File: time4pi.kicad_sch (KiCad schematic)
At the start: 17 parts, among them J1 Raspberry_Pi_2_3, J2 Conn_02x03_Odd_Even, J3 Conn_Coaxial_Small, J4 Conn_Coaxial_Small, J5 RFShield_OnePiece, Q3 BFR92, Q4 BFR92, U1 ECOC 7050, U2 HMC361S8G/361S8GE, U3 ADF4158, U4 AB0805

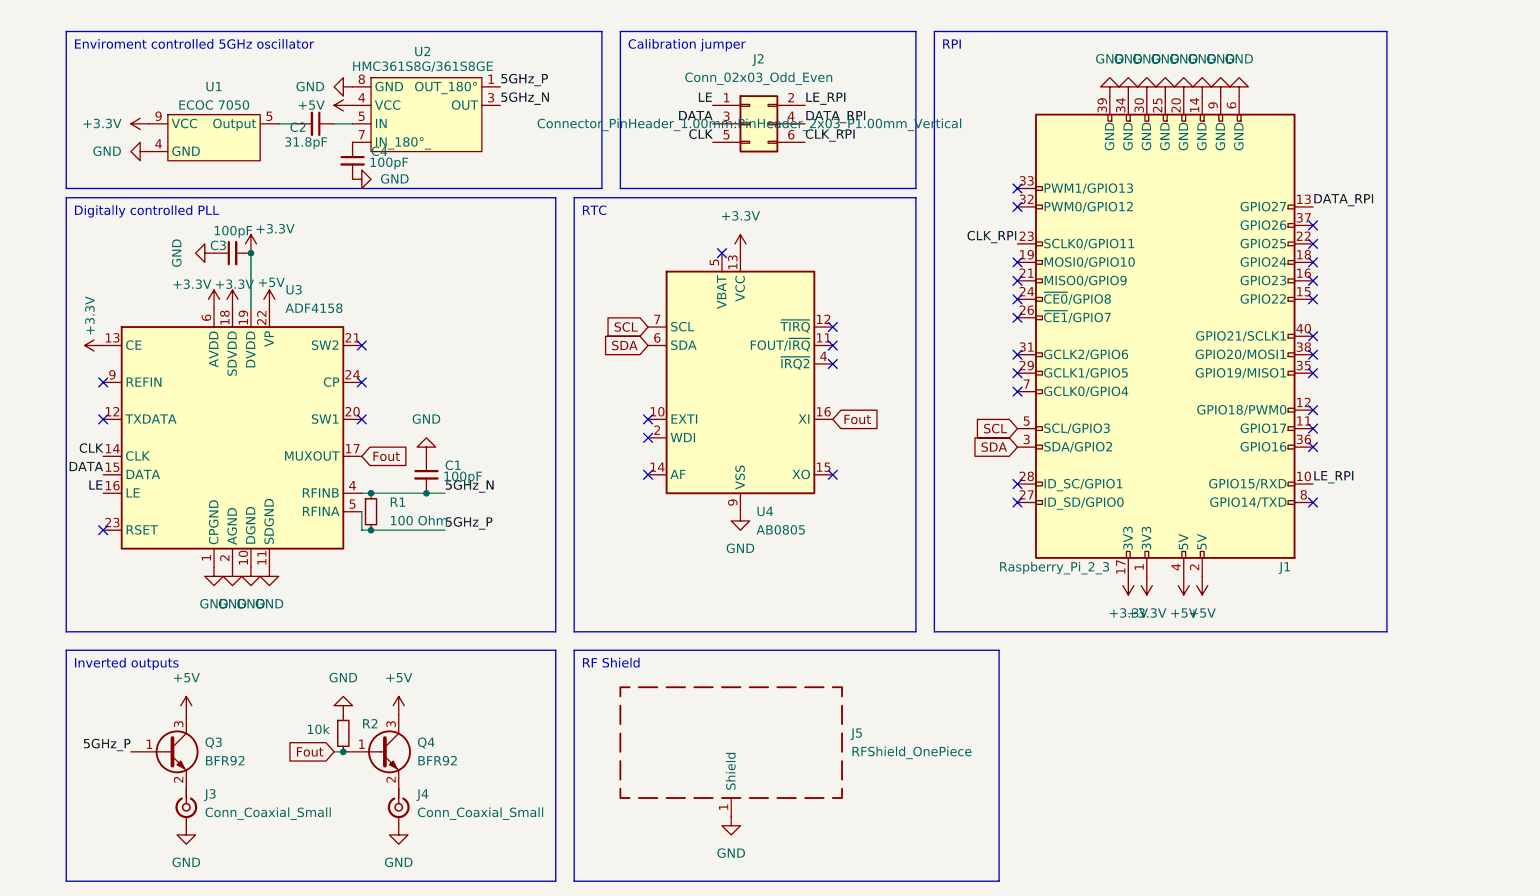
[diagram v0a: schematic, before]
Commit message: feat: more caps
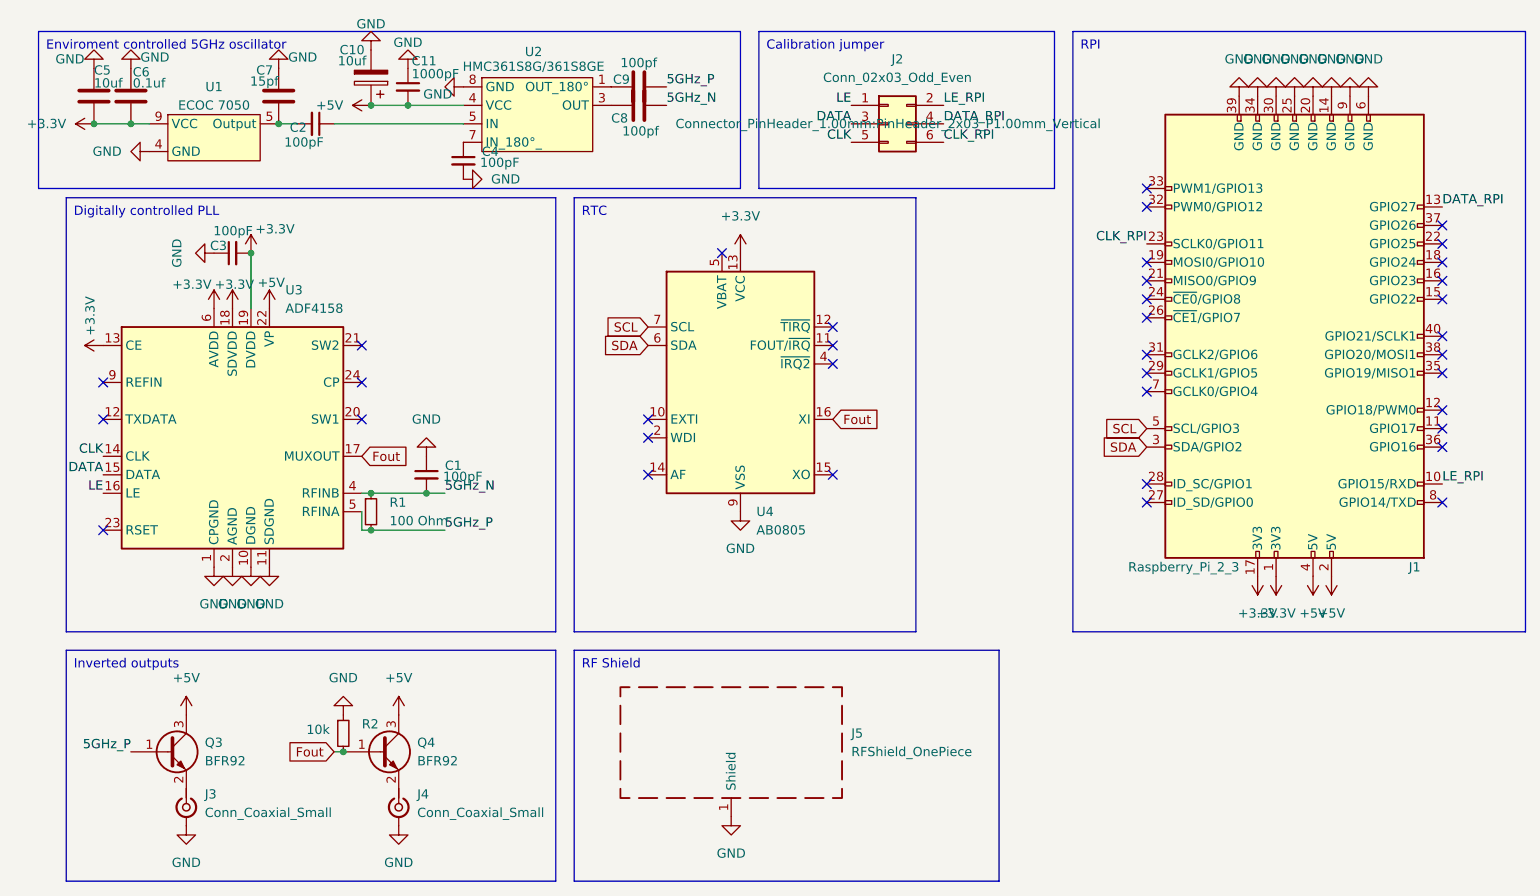
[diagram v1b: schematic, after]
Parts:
- added C10: 10uf, Capacitor_SMD:CP_Elec_4x3, symbol Device:C_Polarized
- added C11: 1000pF, Capacitor_SMD:C_0201_0603Metric, symbol Device:C_Small
- added C5: 10uf, Capacitor_SMD:C_0201_0603Metric, symbol Device:C
- added C6: 0.1uf, Capacitor_SMD:C_0201_0603Metric, symbol Device:C
- added C7: 15pf, Capacitor_SMD:C_0201_0603Metric, symbol Device:C
- added C8, C9: 100pf, Capacitor_SMD:C_0201_0603Metric, symbol Device:C
- C2: value 31.8pF -> 100pF
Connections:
- net +3.3V: now also C5.2, C6.2
- net +5V: now also C10.1, C11.2
- net 5GHz_N: now also C8.1; no longer U2.3 (OUT)
- net 5GHz_P: now also C9.1; no longer U2.1 (OUT_180°)
- net GND: now also C10.2, C11.1, C5.1, C6.1, C7.2
- net at C2.2, U1.5 (Output): now also C7.1
- new net: C8.2, U2.3 (OUT)
- new net: C9.2, U2.1 (OUT_180°)
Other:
- moved on the sheet: C4, J1, J2, U2
